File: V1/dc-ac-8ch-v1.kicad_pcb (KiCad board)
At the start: 2 copper layers, 98 x 67.8 mm, 103 parts, among them J1 DB142V-5.08-4P, J2 DB142V-5.08-4P, J3 DB142V-5.08-2P, J4 DB142V-5.08-4P, J5 DB142V-5.08-4P, J6 DB142V-5.08-2P, U1 MOC3063S, U2 MOC3063S, U3 MOC3063S, U4 MOC3063S, U5 MOC3063S, U6 MOC3063S, U7 MOC3063S, U8 MOC3063S

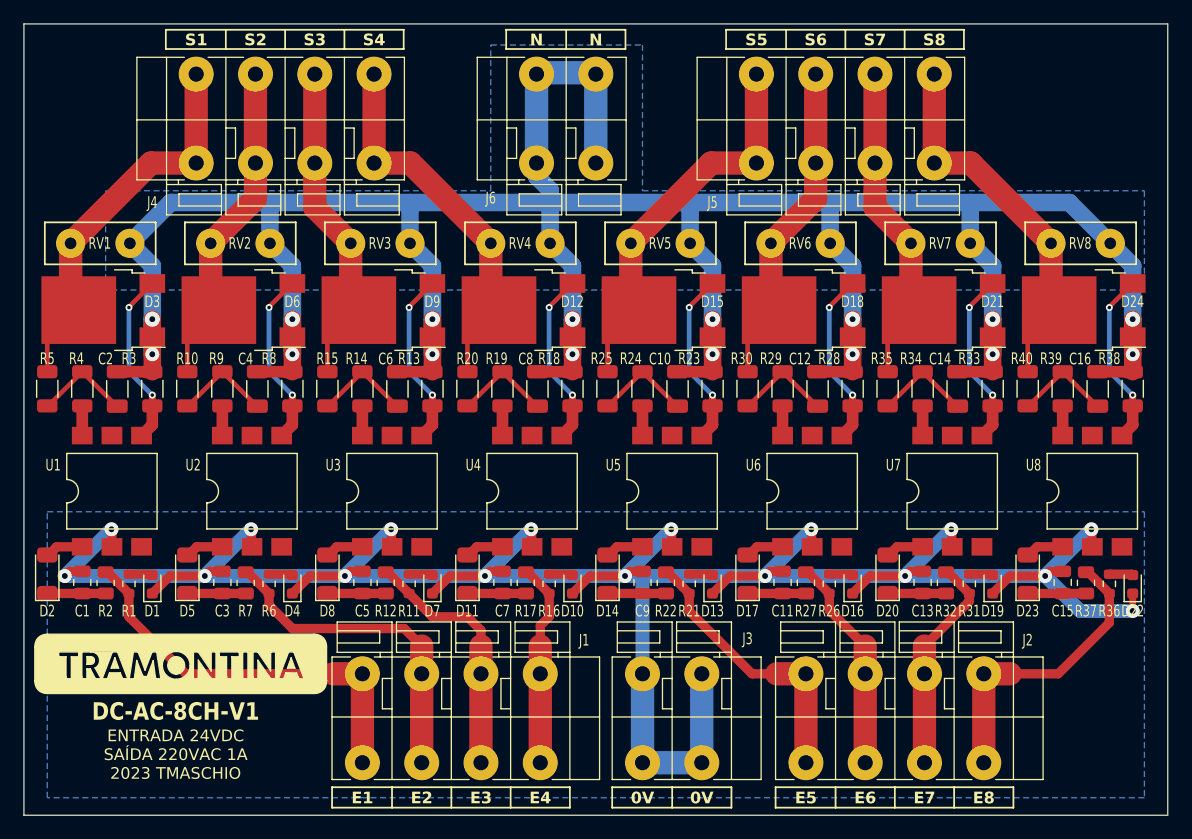
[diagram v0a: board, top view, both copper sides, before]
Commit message: Update dc-ac-8ch-v1.kicad_pcb
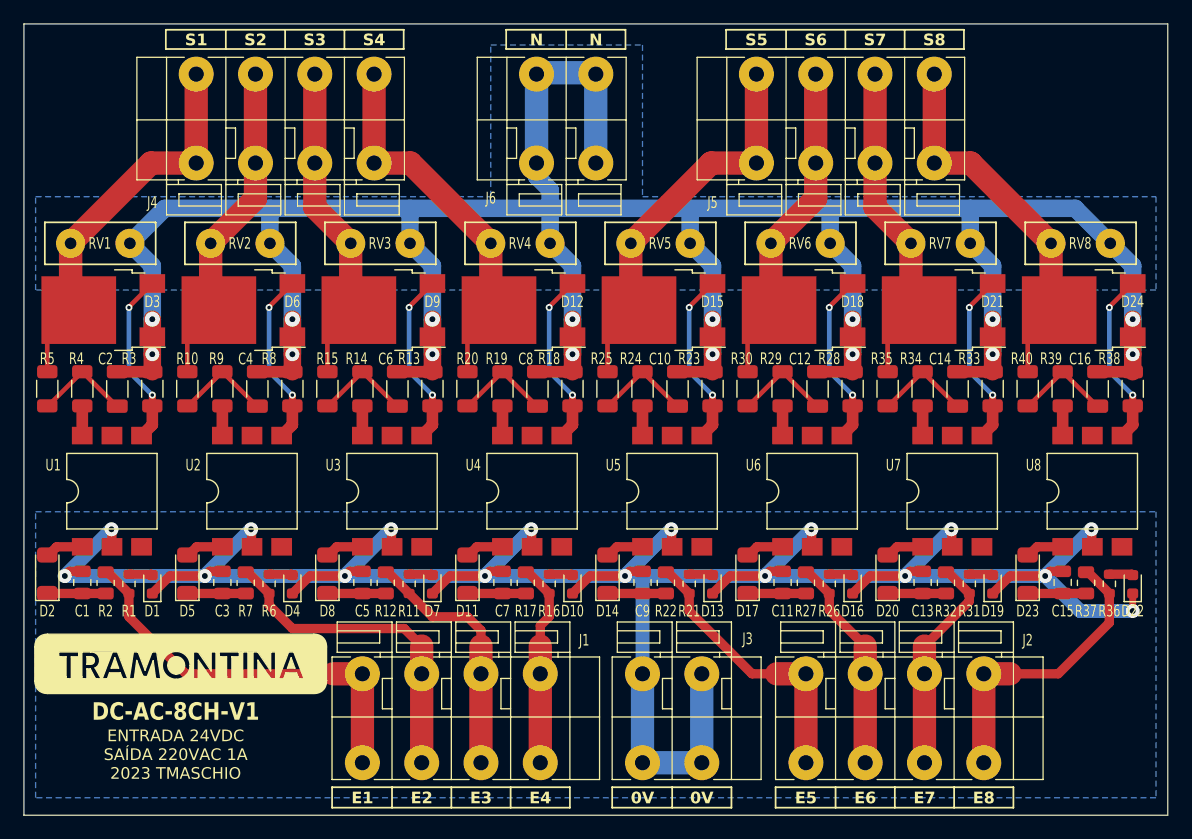
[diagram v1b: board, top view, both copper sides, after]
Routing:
- net NEUTRAL: track 274.9 -> 272.0 mm
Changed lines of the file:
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@@
   (segment (start 143.92 74) (end 143.92 66.38) (width 2) (layer "B.Cu") (net 4))
   (segment (start 183 87.5) (end 183 82.92) (width 1.5) (layer "B.Cu") (net 4))
+  (segment (start 169.08 81) (end 169.08 78) (width 1.5) (layer "B.Cu") (net 4))
   (segment (start 145.08 76.42) (end 143.92 75.26) (width 1.5) (layer "B.Cu") (net 4))
+  (segment (start 121.08 81) (end 121.08 78) (width 1.5) (layer "B.Cu") (net 4))
   (segment (start 195 82.92) (end 193.08 81) (width 1.5) (layer "B.Cu") (net 4))
-  (segment (start 189.58 77.5) (end 193.08 81) (width 1.5) (layer "B.Cu") (net 4))
-  (segment (start 181.08 81) (end 181.08 77.5) (width 1.5) (layer "B.Cu") (net 4))
+  (segment (start 109.08 81) (end 112.08 78) (width 1.5) (layer "B.Cu") (net 4))
   (segment (start 135 87.5) (end 135 90.5) (width 1.5) (layer "B.Cu") (net 4))
-  (segment (start 133.08 81) (end 133.08 77.5) (width 1.5) (layer "B.Cu") (net 4))
   (segment (start 147 87.5) (end 147 90.5) (width 1.5) (layer "B.Cu") (net 4))
   (segment (start 159 87.5) (end 159 90.5) (width 1.5) (layer "B.Cu") (net 4))
   (segment (start 171 87.5) (end 171 90.5) (width 1.5) (layer "B.Cu") (net 4))
-  (segment (start 157.08 81) (end 157.08 77.5) (width 1.5) (layer "B.Cu") (net 4))
   (segment (start 183 87.5) (end 183 90.5) (width 1.5) (layer "B.Cu") (net 4))
   (segment (start 171 87.5) (end 171 82.92) (width 1.5) (layer "B.Cu") (net 4))
   (segment (start 195 87.5) (end 195 82.92) (width 1.5) (layer "B.Cu") (net 4))
-  (segment (start 112.58 77.5) (end 189.58 77.5) (width 1.5) (layer "B.Cu") (net 4))
   (segment (start 147 82.92) (end 145.08 81) (width 1.5) (layer "B.Cu") (net 4))
   (segment (start 159 87.5) (end 159 82.92) (width 1.5) (layer "B.Cu") (net 4))
   (segment (start 159 82.92) (end 157.08 81) (width 1.5) (layer "B.Cu") (net 4))
-  (segment (start 109.08 81) (end 112.58 77.5) (width 1.5) (layer "B.Cu") (net 4))
-  (segment (start 169.08 81) (end 169.08 77.5) (width 1.5) (layer "B.Cu") (net 4))
+  (segment (start 133.08 81) (end 133.08 78) (width 1.5) (layer "B.Cu") (net 4))
   (segment (start 123 82.92) (end 121.08 81) (width 1.5) (layer "B.Cu") (net 4))
+  (segment (start 190.08 78) (end 193.08 81) (width 1.5) (layer "B.Cu") (net 4))
   (segment (start 123 87.5) (end 123 82.92) (width 1.5) (layer "B.Cu") (net 4))
   (segment (start 123 87.5) (end 123 90.5) (width 1.5) (layer "B.Cu") (net 4))
@@
   (segment (start 145.08 81) (end 145.08 76.42) (width 1.5) (layer "B.Cu") (net 4))
   (segment (start 147 87.5) (end 147 82.92) (width 1.5) (layer "B.Cu") (net 4))
-  (segment (start 121.08 81) (end 121.08 77.5) (width 1.5) (layer "B.Cu") (net 4))
+  (segment (start 181.08 81) (end 181.08 78) (width 1.5) (layer "B.Cu") (net 4))
+  (segment (start 157.08 81) (end 157.08 78) (width 1.5) (layer "B.Cu") (net 4))
   (segment (start 149 74) (end 149 66.38) (width 2) (layer "B.Cu") (net 4))
   (segment (start 111 87.5) (end 111 90.5) (width 1.5) (layer "B.Cu") (net 4))
+  (segment (start 112.08 78) (end 190.08 78) (width 1.5) (layer "B.Cu") (net 4))
   (segment (start 135 82.92) (end 133.08 81) (width 1.5) (layer "B.Cu") (net 4))
   (segment (start 195 87.5) (end 195 90.5) (width 1.5) (layer "B.Cu") (net 4))
@@
     (polygon
       (pts
-        (xy 107 85)
-        (xy 107 76.5)
-        (xy 140 76.5)
+        (xy 101 85)
+        (xy 101 77)
+        (xy 140 77)
         (xy 140 64)
         (xy 153 64)
-        (xy 153 76.5)
-        (xy 196 76.5)
-        (xy 196 85)
+        (xy 153 77)
+        (xy 197 77)
+        (xy 197 85)
       )
     )
@@
     (polygon
       (pts
-        (xy 102 104)
-        (xy 196 104)
-        (xy 196 128.5)
-        (xy 102 128.5)
+        (xy 101 104)
+        (xy 197 104)
+        (xy 197 128.5)
+        (xy 101 128.5)
       )
     )
